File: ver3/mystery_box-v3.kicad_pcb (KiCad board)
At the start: 2 copper layers, 136 x 100 mm, 32 parts, among them J10 Screw_Terminal_01x02, J11 Screw_Terminal_01x02, J12 Screw_Terminal_01x02, J13 Screw_Terminal_01x02, J14 Screw_Terminal_01x02, J15 Screw_Terminal_01x02, J16 Screw_Terminal_01x02, J17 Screw_Terminal_01x02, J18 Barrel_Jack_MountingPin, J20 rj45-CC-X2-Aliexpress, J8 Screw_Terminal_01x02, J9 Screw_Terminal_01x02, Q1 IRLZ44N, Q2 IRLZ44N, Q3 IRLZ44N, U2 MAX485E

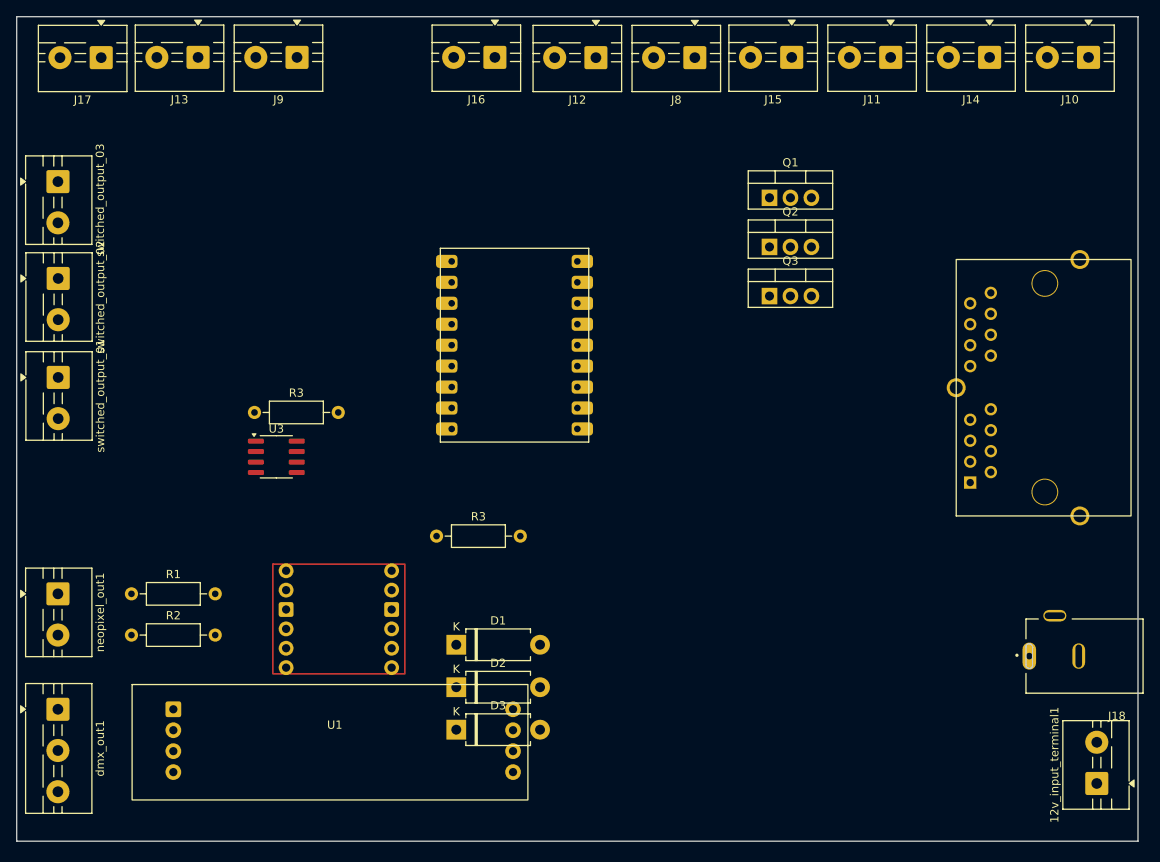
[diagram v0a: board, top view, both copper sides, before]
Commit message: final prototype v3
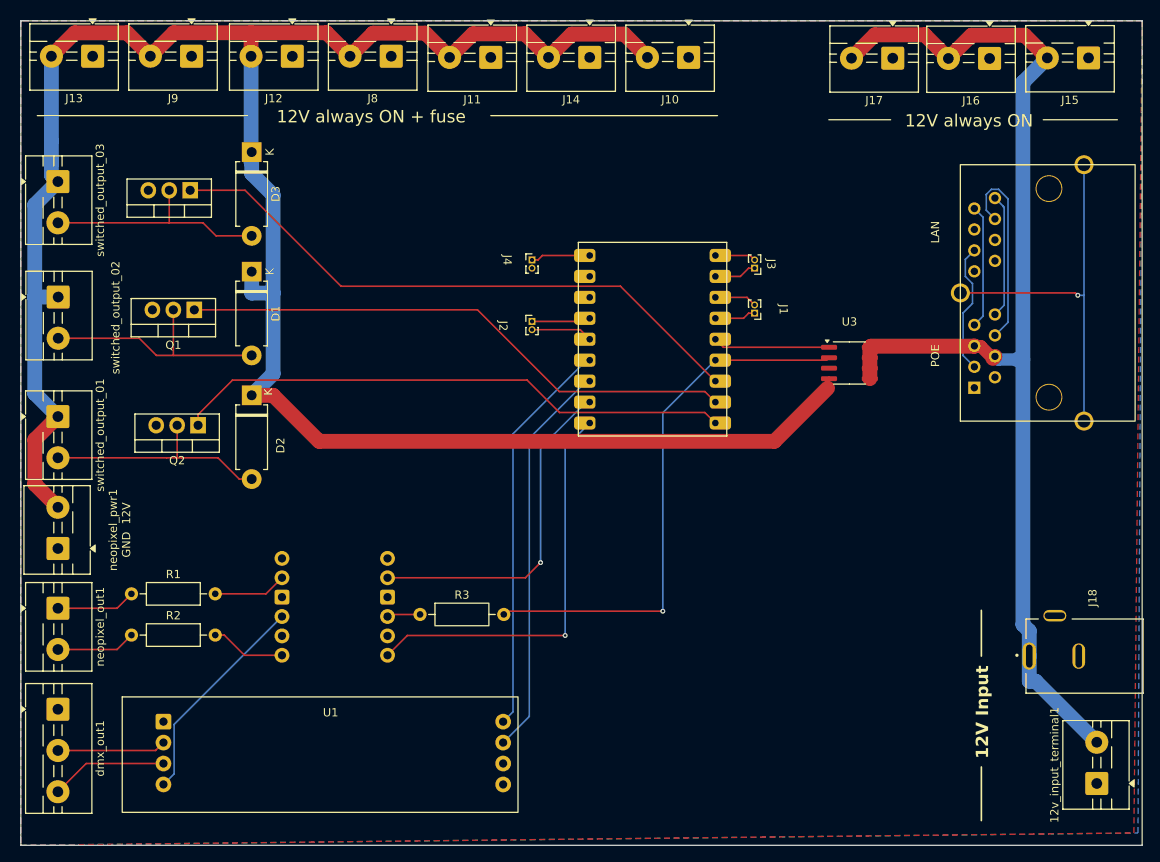
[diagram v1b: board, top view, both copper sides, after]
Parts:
- removed the R3 at (116.8, 78.0)
- removed the R3 at (138.9, 93.0)
- added G***: LOGO, LOGO, F.Cu at (183.5, 112.5)
- added J1: Conn_01x02_Pin, Connector_PinHeader_1.00mm:PinHeader_1x02_P1.00mm_Vertical, F.Cu at (177.5, 66.0)
- added J2: Conn_01x02_Pin, Connector_PinHeader_1.00mm:PinHeader_1x02_P1.00mm_Vertical, F.Cu at (150.5, 67.0)
- added J3: Conn_01x02_Pin, Connector_PinHeader_1.00mm:PinHeader_1x02_P1.00mm_Vertical, F.Cu at (177.5, 60.5)
- added J4: Conn_01x02_Pin, Connector_PinHeader_1.00mm:PinHeader_1x02_P1.00mm_Vertical, F.Cu at (150.5, 59.5)
- added R3: R, Resistor_THT:R_Axial_DIN0207_L6.3mm_D2.5mm_P10.16mm_Horizontal, F.Cu at (136.9, 102.5)
- added neopixel_pwr1 GND  12V: Screw_Terminal_01x02, TerminalBlock:TerminalBlock_MaiXu_MX126-5.0-02P_1x02_P5.00mm, F.Cu at (93.0, 94.5)
- moved J17 96.0 mm to (194.2, 35.0)
- moved D3 74.3 mm to (116.5, 46.4), turned to -90 degrees
- moved Q2 72.6 mm to (110.0, 79.6), turned to 180 degrees
- moved Q3 71.4 mm to (109.0, 51.1), turned to 180 degrees
- moved Q1 71.1 mm to (109.5, 65.6), turned to 180 degrees
- moved U3 70.4 mm to (189.0, 72.0)
- moved J16 60.0 mm to (206.0, 35.1)
- moved D1 51.6 mm to (116.5, 60.9), turned to -90 degrees
- moved J10 48.5 mm to (169.5, 34.9)
- moved J11 48.5 mm to (145.5, 34.9)
- moved J14 48.5 mm to (157.5, 34.9)
- moved D2 43.2 mm to (116.5, 75.9), turned to -90 degrees
- moved J12 36.8 mm to (121.4, 34.8)
- moved J8 36.8 mm to (133.4, 34.8)
- moved J15 36.0 mm to (218.0, 35.0)
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- renumbered ESP32_S1 to ESP32_S3
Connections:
- net Net-(D1-K) renamed /SW 12V
- ESP32_S3 pad 1: (no net) -> Net-(J2-Pin_1)
- ESP32_S3 pad 10: (no net) -> Net-(U3-ST)
- ESP32_S3 pad 11: (no net) -> Net-(U3-IN)
- ESP32_S3 pad 12: (no net) -> Net-(J1-Pin_1)
- ESP32_S3 pad 13: (no net) -> Net-(J1-Pin_2)
- ESP32_S3 pad 2: (no net) -> Net-(J2-Pin_2)
- ESP32_S3 pad 3: (no net) -> Net-(U2-DI)
- ESP32_S3 pad 3V3: (no net) -> unconnected-(ESP32_S3-3.3V(OUT)-Pad3V3)
- ESP32_S3 pad 4: (no net) -> Net-(U2-DE)
- ESP32_S3 pad 5: (no net) -> Net-(U1-LV3)
- ESP32_S3 pad 5V: (no net) -> Net-(J4-Pin_1)
- ESP32_S3 pad 6: (no net) -> Net-(U1-LV1)
- ESP32_S3 pad 7: (no net) -> Net-(Q2-G)
- ESP32_S3 pad 8: (no net) -> Net-(Q1-G)
- ESP32_S3 pad 9: (no net) -> Net-(Q3-G)
- ESP32_S3 pad GND: (no net) -> GND
- ESP32_S3 pad RX: (no net) -> Net-(J3-Pin_1)
- ESP32_S3 pad TX: (no net) -> Net-(J3-Pin_2)
- Q1 pad 1: Net-(ESP32_S1-8) -> Net-(Q1-G)
- Q2 pad 1: Net-(ESP32_S1-7) -> Net-(Q2-G)
- Q3 pad 1: Net-(ESP32_S1-9) -> Net-(Q3-G)
- U1 pad 1: Net-(ESP32_S1-6) -> Net-(U1-LV1)
- U1 pad 5: Net-(ESP32_S1-5) -> Net-(U1-LV3)
- U2 pad 3: Net-(ESP32_S1-4) -> Net-(U2-DE)
- U2 pad 4: Net-(ESP32_S1-3) -> Net-(U2-DI)
- U3 pad 1: Net-(ESP32_S1-11) -> Net-(U3-IN)
- U3 pad 2: Net-(ESP32_S1-10) -> Net-(U3-ST)
- U3 pad 5: VCC -> VCC 12V
- U3 pad 6: VCC -> VCC 12V
- U3 pad 7: VCC -> VCC 12V
- U3 pad 8: VCC -> VCC 12V
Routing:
- net /SW 12V: track 0.00 -> 275.3 mm
- net VCC 12V: track 0.00 -> 140.2 mm
- net Net-(Q3-G): track 0.00 -> 73.3 mm
- net Net-(Q2-G): track 0.00 -> 67.9 mm
- net Net-(Q1-G): track 0.00 -> 67.8 mm
- net Net-(U3-ST): track 0.00 -> 66.4 mm, vias 0 -> 1
- net Net-(U1-LV1): track 0.00 -> 49.5 mm, vias 0 -> 1
- net Net-(U2-DE): track 0.00 -> 48.4 mm
- net Net-(U2-DI): track 0.00 -> 48.4 mm
- net unconnected-(J20-PadSH): track 0.00 -> 46.2 mm, vias 0 -> 1
- net Net-(U1-LV3): track 0.00 -> 41.5 mm, vias 0 -> 1
- net Net-(D1-A): track 0.00 -> 29.9 mm
- net Net-(D2-A): track 0.00 -> 28.5 mm
- net Net-(D3-A): track 0.00 -> 28.1 mm
- net VCC 5V: track 0.00 -> 26.3 mm
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- added copper zone on B.Cu, net GND
- added copper zone on F.Cu, net GND
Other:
- board text added: "12V Input"
- board text added: "12V always ON"
- board text added: "12V always ON + fuse"
- board text added: "Cosmic Cable Ltd. Mysterious Prototype v3"
- board text added: "LAN"
- board text added: "POE"
